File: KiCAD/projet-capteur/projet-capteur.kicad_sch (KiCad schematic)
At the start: 20 parts, among them J1 Power, J2 Analog, J3 Digital/PWM, J4 Digital/PWM, U2 LTC1050

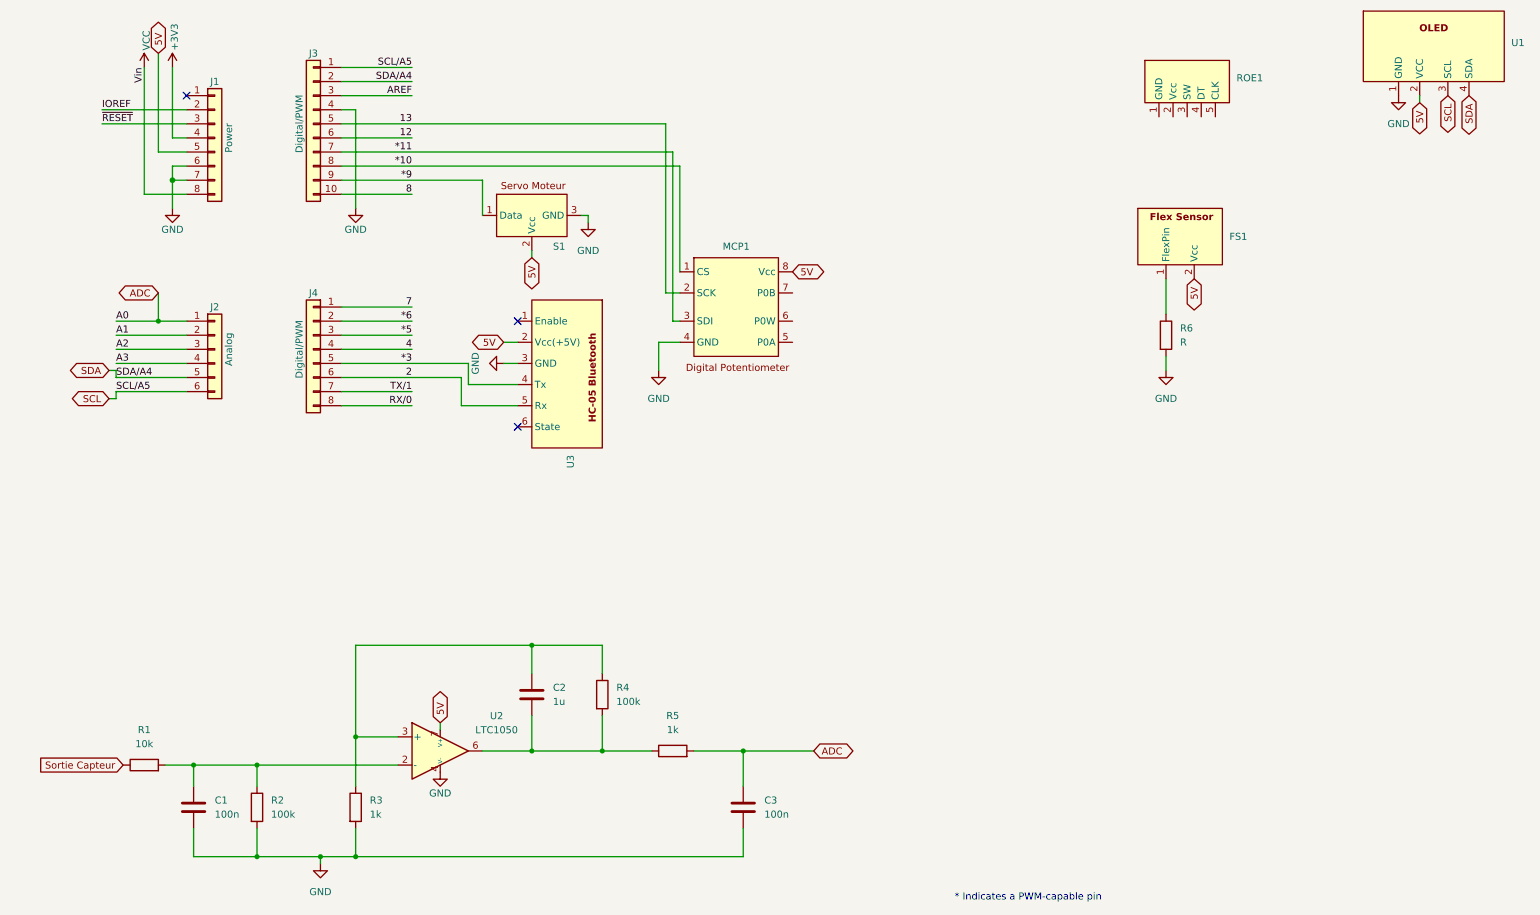
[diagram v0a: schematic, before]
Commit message: Seance Realisation du shield 12.03 v2
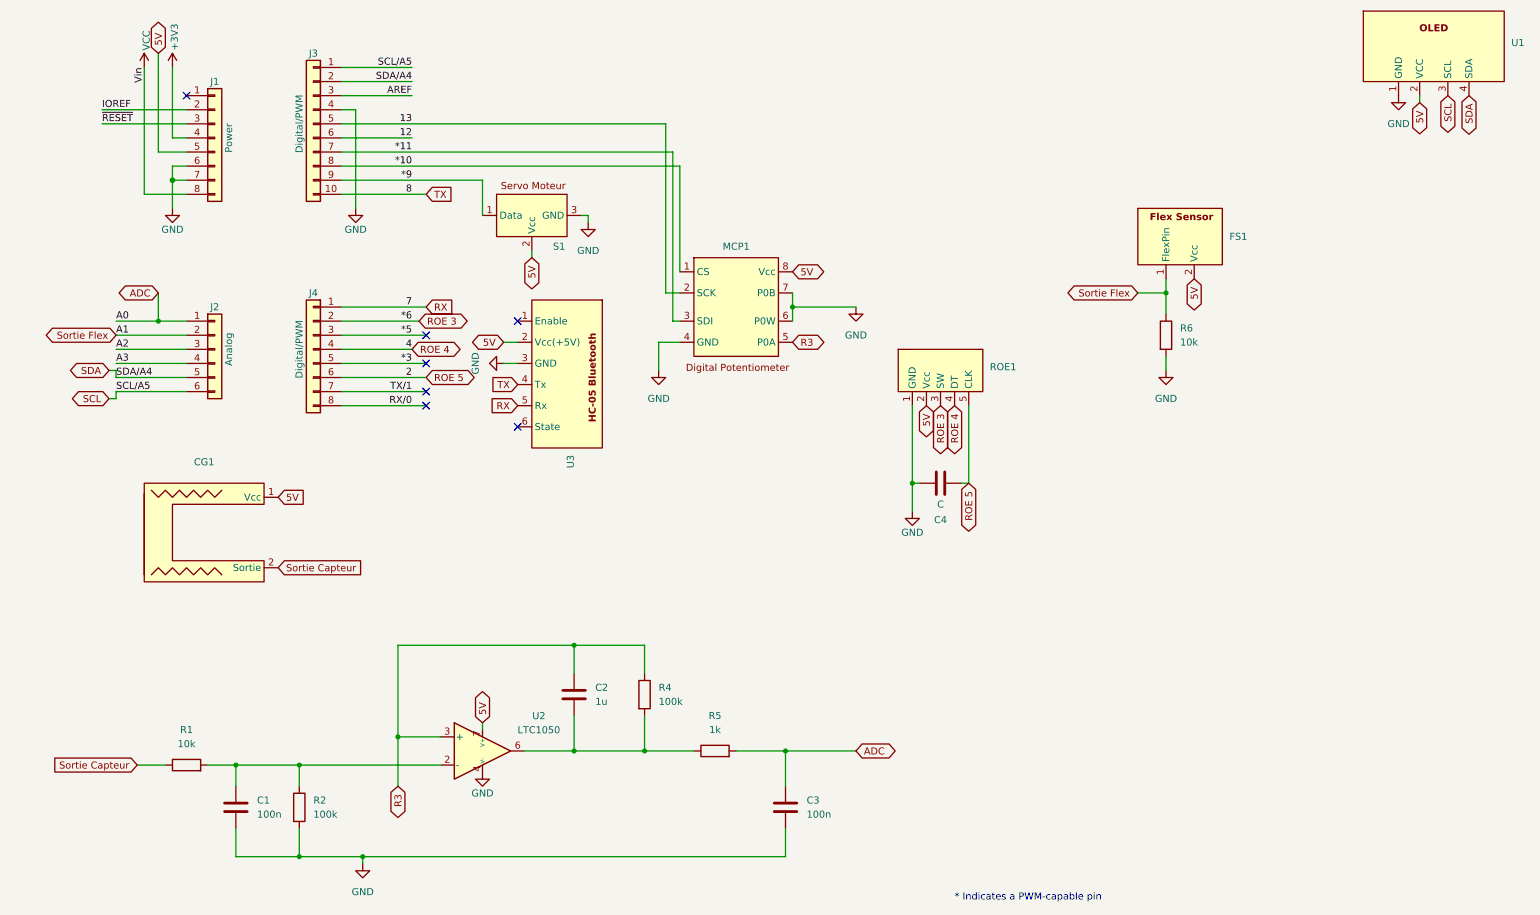
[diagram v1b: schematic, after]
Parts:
- removed R3: 1k, Resistor_THT:R_Axial_DIN0207_L6.3mm_D2.5mm_P5.08mm_Vertical, symbol Device:R
- added C4: C, Capacitor_THT:C_Disc_D6.0mm_W2.5mm_P5.00mm, symbol Device:C
- added CG1: ~, MyLibEmpreinte:Capteur Graphene, symbol MyLibGraphite:Capteur
- R6: value R -> 10k
- ROE1: footprint MyLibEmpreinte:Rotary Encoder -> MyLibEmpreinte:RotaryEncoder
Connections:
- net *6 is gone; now on net ROE 3: J4.2 (Pin_2)
- net 4 is gone; now on net ROE 4: J4.4 (Pin_4)
- net 7 is gone; now on net RX: J4.1 (Pin_1)
- net A1 is gone; now on net Sortie Flex: J2.2 (Pin_2)
- net *3: no longer U3.4 (Tx)
- net 5V: now also ROE1.2 (Vcc), CG1.1 (Vcc)
- net GND: now also MCP1.6 (P0W), MCP1.7 (P0B), ROE1.1 (GND), C4.1
- net Sortie Capteur: now also CG1.2 (Sortie)
- net Sortie Flex: now reaches FS1.1 (FlexPin), R6.1
- net R3: now reaches C2.1, R4.1, U2.3 (+)
- net R3: now also MCP1.5 (P0A)
- net ROE 3: now reaches ROE1.3 (SW)
- net ROE 4: now reaches ROE1.4 (DT)
- net ROE 5: now reaches ROE1.5 (CLK)
- net ROE 5: now also J4.6 (Pin_6), C4.2
- net 2 renamed RX
- net RX: no longer J4.6 (Pin_6)
- net 8 renamed TX
- net TX: now also U3.4 (Tx)
- no-connect marks 3 -> 7
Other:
- moved on the sheet: C1, C2, C3, R1, R2, R4, R5, ROE1, U2
